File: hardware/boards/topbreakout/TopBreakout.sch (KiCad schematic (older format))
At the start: 0 parts

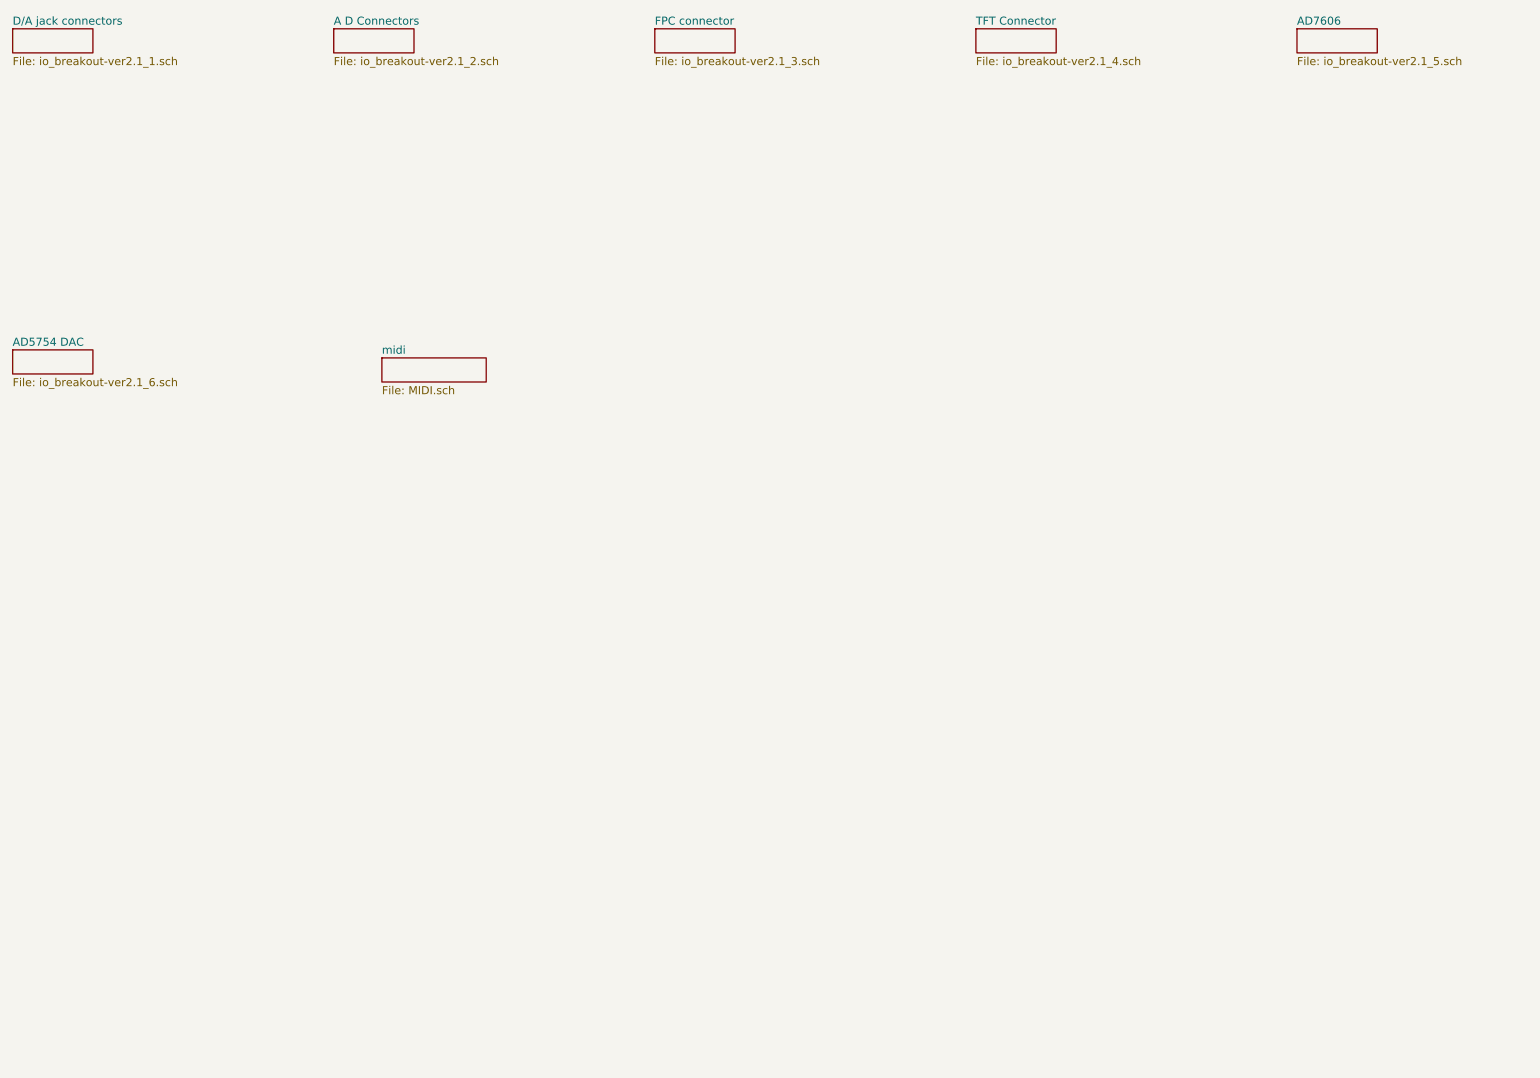
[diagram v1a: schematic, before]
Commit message: mainboard v1.7
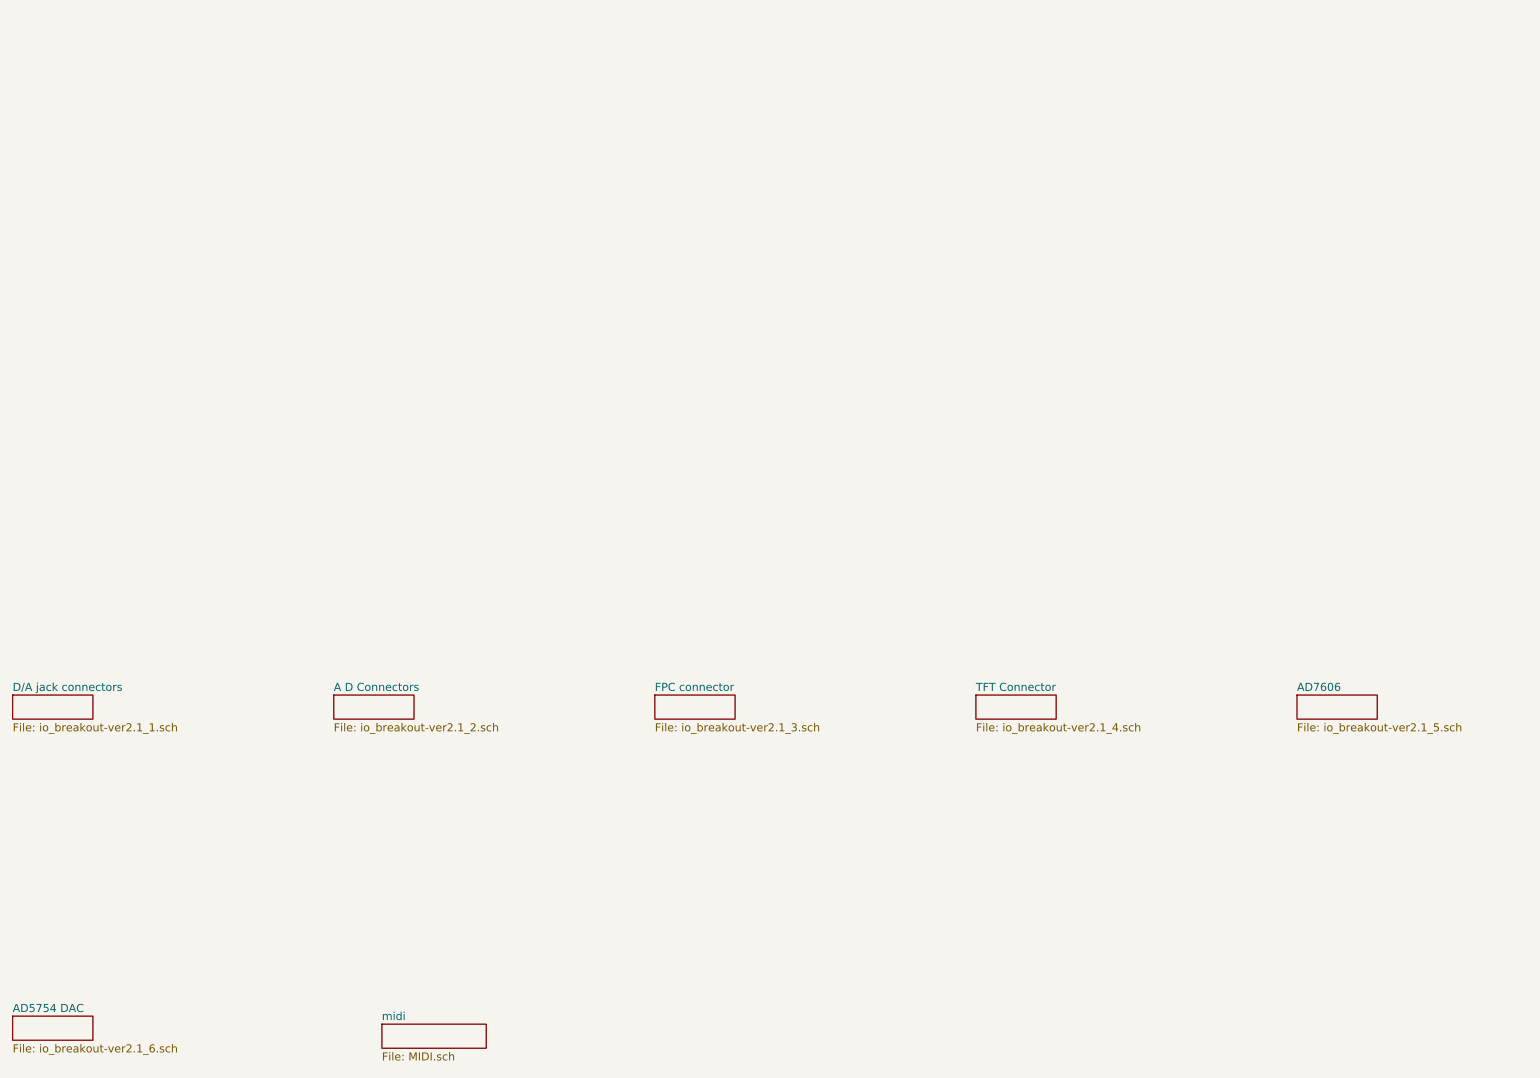
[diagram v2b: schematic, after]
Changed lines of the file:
@@
-EESchema Schematic File Version 5
+EESchema Schematic File Version 4
 EELAYER 30 0
 EELAYER END
@@
 Comment3 ""
 Comment4 ""
-Comment5 ""
-Comment6 ""
-Comment7 ""
-Comment8 ""
-Comment9 ""
 $EndDescr
 $Sheet
-S 1000 1000 500  150
+S 1000 5150 500  150
 U 5D7F4208
 F0 "D/A jack connectors" 50
@@
 $EndSheet
 $Sheet
-S 3000 1000 500  150
+S 3000 5150 500  150
 U 5D7F4281
 F0 "A D Connectors" 50
@@
 $EndSheet
 $Sheet
-S 5000 1000 500  150
+S 5000 5150 500  150
 U 5D7F42FA
 F0 "FPC connector" 50
@@
 $EndSheet
 $Sheet
-S 7000 1000 500  150
+S 7000 5150 500  150
 U 5D7F4364
 F0 "TFT Connector" 50
@@
 $EndSheet
 $Sheet
-S 9000 1000 500  150
+S 9000 5150 500  150
 U 5D7F4383
 F0 "AD7606" 50
@@
 $EndSheet
 $Sheet
-S 1000 3000 500  150
+S 1000 7150 500  150
 U 5D7F4465
 F0 "AD5754 DAC" 50
@@
 $EndSheet
 $Sheet
-S 3300 3050 650  150
+S 3300 7200 650  150
 U 5D8CF794
 F0 "midi" 50
